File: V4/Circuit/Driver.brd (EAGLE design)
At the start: 58.1 x 81.3 mm, 54 parts, among them IC1 DRV8303DCA

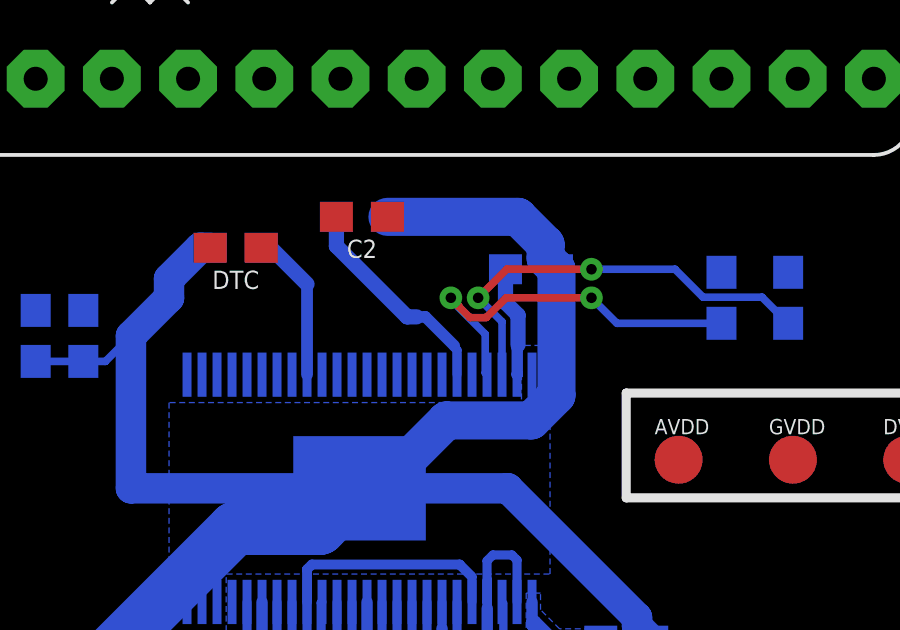
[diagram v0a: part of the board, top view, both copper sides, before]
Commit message: Ready for V4 autoroutering 4
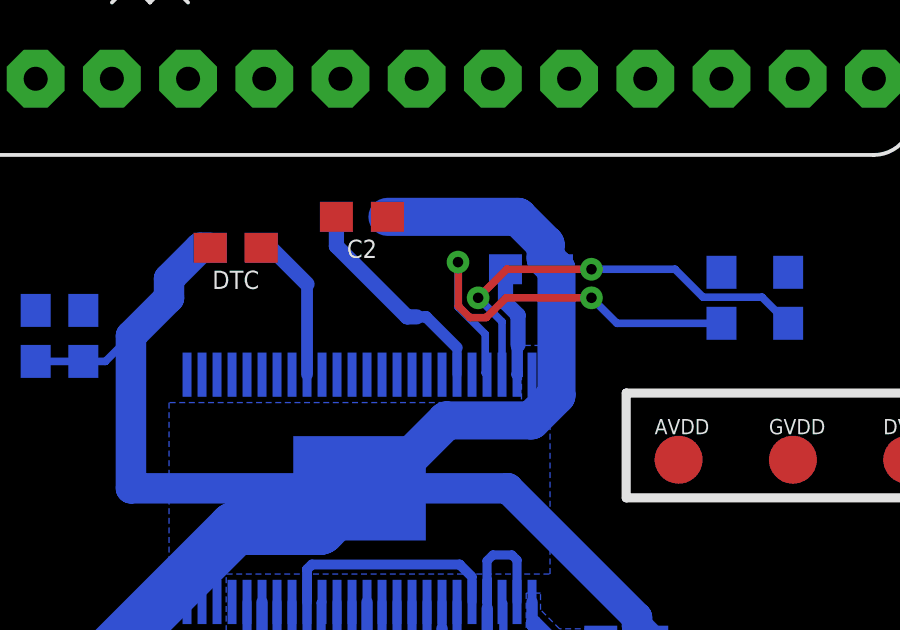
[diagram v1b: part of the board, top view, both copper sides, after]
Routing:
- net SO1B: track 13.0 -> 15.2 mm
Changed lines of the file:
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@@
 <wire x1="34.789375" y1="57.30875" x2="34.789375" y2="56.333125" width="0.508" layer="16"/>
 <wire x1="37.1475" y1="53.975" x2="37.465" y2="53.975" width="0.508" layer="16"/>
-<wire x1="38.694525" y1="52.982025" x2="38.81" y2="52.86655" width="0.3048" layer="16"/>
-<wire x1="38.81" y1="52.86655" x2="38.81" y2="52.048" width="0.3048" layer="16"/>
 <wire x1="34.789375" y1="56.333125" x2="37.1475" y2="53.975" width="0.508" layer="16"/>
-<wire x1="37.465" y1="53.975" x2="37.75543125" y2="53.975" width="0.381" layer="16"/>
-<wire x1="37.75543125" y1="53.975" x2="38.721465625" y2="53.008965625" width="0.381" layer="16"/>
+<wire x1="37.465" y1="53.975" x2="37.7825" y2="53.975" width="0.381" layer="16"/>
+<wire x1="38.81" y1="52.9475" x2="38.81" y2="52.048" width="0.3048" layer="16"/>
+<wire x1="37.7825" y1="53.975" x2="38.81" y2="52.9475" width="0.381" layer="16"/>
 <wire x1="38.81" y1="52.048" x2="53.81625" y2="49.2125" width="0" layer="19" extent="1-16"/>
-<wire x1="38.721465625" y1="53.008965625" x2="38.694525" y2="52.982025" width="0" layer="19" extent="16-16"/>
 </signal>
 <signal name="SO1">
@@
 <contactref element="IC1" pad="21"/>
 <contactref element="R5" pad="2"/>
-<via x="38.60425625" y="54.61" extent="1-16" drill="0.35"/>
-<wire x1="38.60425625" y1="54.5450625" x2="38.60425625" y2="54.61" width="0.254" layer="16"/>
-<wire x1="39.7498" y1="53.39951875" x2="38.60425625" y2="54.5450625" width="0.254" layer="16"/>
+<via x="38.84238125" y="55.800625" extent="1-16" drill="0.35"/>
+<wire x1="38.84238125" y1="54.3069375" x2="38.84238125" y2="55.800625" width="0.254" layer="16"/>
+<wire x1="39.7498" y1="53.39951875" x2="38.84238125" y2="54.3069375" width="0.254" layer="16"/>
 <wire x1="39.81" y1="52.048" x2="39.7498" y2="52.1082" width="0.254" layer="16"/>
 <wire x1="39.7498" y1="52.1082" x2="39.7498" y2="53.39951875" width="0.254" layer="16"/>
@@
 <wire x1="39.24066875" y1="53.9524" x2="38.85545625" y2="54.3376125" width="0.254" layer="1"/>
 <wire x1="43.2906" y1="54.61" x2="40.44304375" y2="54.61" width="0.254" layer="1"/>
-<wire x1="38.85545625" y1="54.3376125" x2="38.85545625" y2="54.3588" width="0.254" layer="1"/>
-<wire x1="38.85545625" y1="54.3588" x2="38.60425625" y2="54.61" width="0.254" layer="1"/>
+<wire x1="38.85545625" y1="54.3376125" x2="38.85545625" y2="55.78755" width="0.254" layer="1"/>
+<wire x1="38.85545625" y1="55.78755" x2="38.84238125" y2="55.800625" width="0.254" layer="1"/>
 <wire x1="40.44304375" y1="54.61" x2="39.78544375" y2="53.9524" width="0.254" layer="1"/>
 </signal>

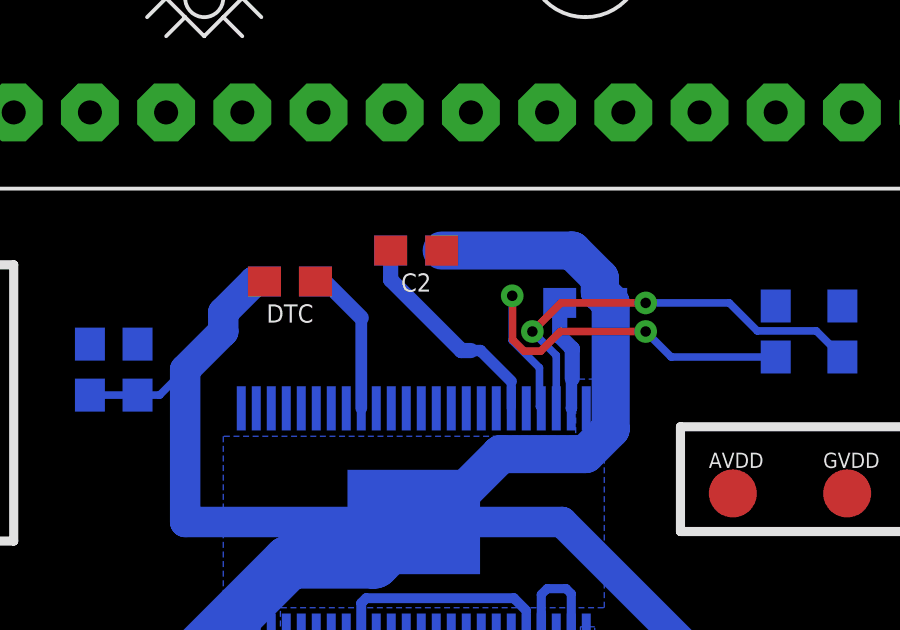
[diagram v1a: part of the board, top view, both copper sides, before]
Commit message: Ready for V4 autoroutering 5
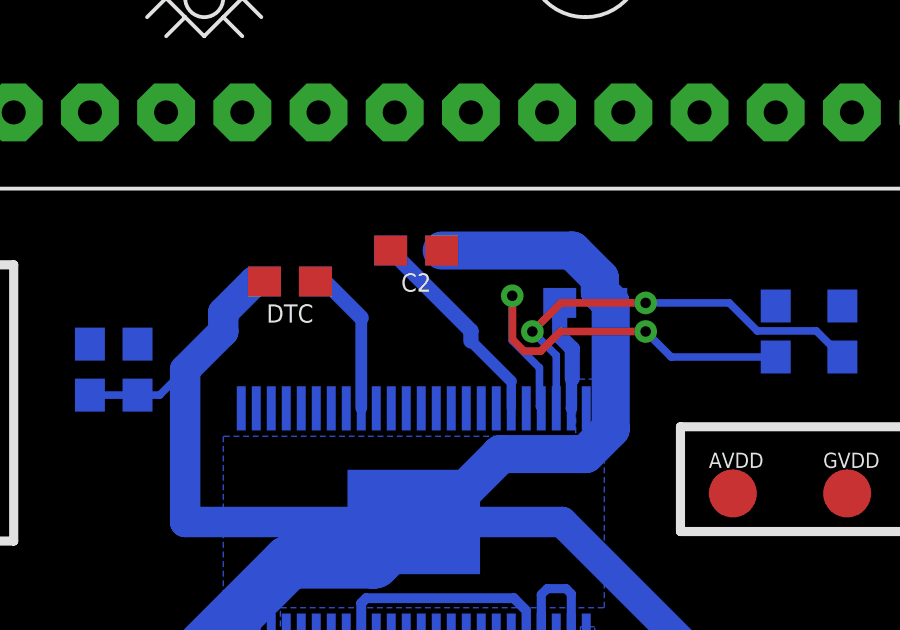
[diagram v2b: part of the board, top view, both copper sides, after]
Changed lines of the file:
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@@
 <wire x1="36.489375" y1="57.30875" x2="40.8423" y2="57.30875" width="1.27" layer="16"/>
 <wire x1="40.8423" y1="57.30875" x2="41.7624" y2="56.38865" width="1.27" layer="16"/>
-<wire x1="42.125" y1="55.5625" x2="50.165" y2="61.9125" width="0" layer="19" extent="16-16"/>
-<wire x1="32.2825" y1="56.276875" x2="30.5825" y2="56.276875" width="0" layer="19" extent="1-16"/>
-<wire x1="3.568" y1="55.245" x2="9.31" y2="39.37" width="0" layer="19" extent="1-1"/>
-<wire x1="4.445" y1="77.1525" x2="3.568" y2="55.245" width="0" layer="19" extent="1-1"/>
-<wire x1="6.985" y1="77.1525" x2="4.445" y2="77.1525" width="0" layer="19" extent="1-1"/>
 </signal>
 <signal name="N$4">
@@
 <contactref element="IC1" pad="45"/>
 <contactref element="IC1" pad="20"/>
-<wire x1="39.31" y1="52.048" x2="52.705" y2="61.9125" width="0" layer="19" extent="16-16"/>
-<wire x1="31.31" y1="44.472" x2="39.31" y2="52.048" width="0" layer="19" extent="16-16"/>
-<wire x1="9.525" y1="77.1525" x2="39.31" y2="52.048" width="0" layer="19" extent="16-16"/>
 </signal>
 <signal name="N$6">
@@
 <wire x1="28.2575" y1="26.035" x2="28.2575" y2="24.9875" width="0.3048" layer="1"/>
 <wire x1="28.2575" y1="24.9875" x2="26.41" y2="23.14" width="0.3048" layer="1"/>
-<wire x1="24.13" y1="2.54" x2="24.13" y2="3.175" width="0" layer="19" extent="1-1"/>
 </signal>
 <signal name="GL_A">
@@
 <contactref element="U$1" pad="P$3"/>
 <contactref element="N_OCTW" pad="TP"/>
-<wire x1="26.3525" y1="54.19" x2="29.81" y2="52.048" width="0" layer="19" extent="16-16"/>
-<wire x1="20.0025" y1="48.815625" x2="26.3525" y2="54.19" width="0" layer="19" extent="1-16"/>
-<wire x1="9.525" y1="61.9125" x2="20.0025" y2="48.815625" width="0" layer="19" extent="1-1"/>
 </signal>
 <signal name="N_FAULT">
@@
 <contactref element="N_FAULT" pad="TP"/>
 <wire x1="7.2" y1="61.9125" x2="6.985" y2="61.9125" width="0.254" layer="16"/>
-<wire x1="24.765" y1="54.19" x2="30.31" y2="52.048" width="0" layer="19" extent="16-16"/>
-<wire x1="9.68375" y1="48.895" x2="24.765" y2="54.19" width="0" layer="19" extent="1-16"/>
-<wire x1="7.2" y1="61.9125" x2="9.68375" y2="48.895" width="0" layer="19" extent="1-16"/>
 </signal>
 <signal name="NSCS">
 <contactref element="IC1" pad="4"/>
 <contactref element="U$1" pad="P$32"/>
-<wire x1="31.31" y1="52.048" x2="32.385" y2="77.1525" width="0" layer="19" extent="16-16"/>
 </signal>
 <signal name="SDI">
 <contactref element="IC1" pad="5"/>
 <contactref element="U$1" pad="P$29"/>
-<wire x1="31.81" y1="52.048" x2="24.765" y2="77.1525" width="0" layer="19" extent="16-16"/>
 </signal>
 <signal name="SDO">
 <contactref element="IC1" pad="6"/>
 <contactref element="U$1" pad="P$30"/>
-<wire x1="32.31" y1="52.048" x2="27.305" y2="77.1525" width="0" layer="19" extent="16-16"/>
 </signal>
 <signal name="SCLK">
 <contactref element="IC1" pad="7"/>
 <contactref element="U$1" pad="P$31"/>
-<wire x1="32.81" y1="52.048" x2="29.845" y2="77.1525" width="0" layer="19" extent="16-16"/>
 </signal>
 <signal name="DC_CAL">
 <contactref element="IC1" pad="8"/>
 <contactref element="U$1" pad="P$12"/>
-<wire x1="33.31" y1="52.048" x2="32.385" y2="61.9125" width="0" layer="19" extent="16-16"/>
 </signal>
 <signal name="GVDD">
@@
 <wire x1="33.81" y1="55.066875" x2="32.6" y2="56.276875" width="0.508" layer="16"/>
 <wire x1="32.2825" y1="56.276875" x2="32.6" y2="56.276875" width="0.508" layer="16"/>
-<wire x1="33.81" y1="52.048" x2="50.00625" y2="49.2125" width="0" layer="19" extent="1-16"/>
 </signal>
 <signal name="N$35">
 <contactref element="IC1" pad="10"/>
 <contactref element="C2" pad="2"/>
-<wire x1="34.31" y1="52.048" x2="34.789375" y2="57.30875" width="0" layer="19" extent="1-16"/>
 </signal>
 <signal name="N$36">
 <contactref element="IC1" pad="11"/>
 <contactref element="C2" pad="1"/>
-<wire x1="34.81" y1="52.048" x2="36.489375" y2="57.30875" width="0" layer="19" extent="1-16"/>
 </signal>
 <signal name="EN_GATE">
@@
 <contactref element="D1" pad="C"/>
 <contactref element="U$1" pad="P$1"/>
-<wire x1="5.322" y1="55.245" x2="35.31" y2="52.048" width="0" layer="19" extent="1-16"/>
-<wire x1="4.445" y1="61.9125" x2="5.322" y2="55.245" width="0" layer="19" extent="1-1"/>
 </signal>
 <signal name="INHA">
@@
 <contactref element="INHA" pad="TP"/>
 <contactref element="U$1" pad="P$5"/>
-<wire x1="14.605" y1="61.9125" x2="35.81" y2="52.048" width="0" layer="19" extent="16-16"/>
-<wire x1="9.525" y1="54.9275" x2="14.605" y2="61.9125" width="0" layer="19" extent="1-1"/>
 </signal>
 <signal name="INLA">
 <contactref element="IC1" pad="14"/>
 <contactref element="U$1" pad="P$14"/>
-<wire x1="36.31" y1="52.048" x2="37.465" y2="61.9125" width="0" layer="19" extent="16-16"/>
 </signal>
 <signal name="INHB">
@@
 <contactref element="INHB" pad="TP"/>
 <contactref element="U$1" pad="P$6"/>
-<wire x1="17.145" y1="61.9125" x2="36.81" y2="52.048" width="0" layer="19" extent="16-16"/>
-<wire x1="14.605" y1="54.9275" x2="17.145" y2="61.9125" width="0" layer="19" extent="1-1"/>
 </signal>
 <signal name="INLB">
 <contactref element="IC1" pad="16"/>
 <contactref element="U$1" pad="P$15"/>
-<wire x1="37.31" y1="52.048" x2="40.005" y2="61.9125" width="0" layer="19" extent="16-16"/>
 </signal>
 <signal name="INHC">
@@
 <contactref element="INHC" pad="TP"/>
 <contactref element="U$1" pad="P$7"/>
-<wire x1="20.0025" y1="54.9275" x2="37.81" y2="52.048" width="0" layer="19" extent="1-16"/>
-<wire x1="19.685" y1="61.9125" x2="20.0025" y2="54.9275" width="0" layer="19" extent="1-1"/>
 </signal>
 <signal name="INLC">
 <contactref element="IC1" pad="18"/>
 <contactref element="U$1" pad="P$16"/>
-<wire x1="38.31" y1="52.048" x2="42.545" y2="61.9125" width="0" layer="19" extent="16-16"/>
 </signal>
 <signal name="DVDD">
@@
 <contactref element="DVDD_CAP" pad="1"/>
 <contactref element="DVDD" pad="TP"/>
-<wire x1="34.789375" y1="57.30875" x2="34.789375" y2="56.333125" width="0.508" layer="16"/>
-<wire x1="37.1475" y1="53.975" x2="37.465" y2="53.975" width="0.508" layer="16"/>
-<wire x1="34.789375" y1="56.333125" x2="37.1475" y2="53.975" width="0.508" layer="16"/>
-<wire x1="37.465" y1="53.975" x2="37.7825" y2="53.975" width="0.381" layer="16"/>
 <wire x1="38.81" y1="52.9475" x2="38.81" y2="52.048" width="0.3048" layer="16"/>
-<wire x1="37.7825" y1="53.975" x2="38.81" y2="52.9475" width="0.381" layer="16"/>
+<wire x1="37.465" y1="54.2925" x2="38.81" y2="52.9475" width="0.381" layer="16"/>
+<wire x1="34.789375" y1="57.30875" x2="37.465" y2="54.633125" width="0.508" layer="16"/>
+<wire x1="37.465" y1="54.633125" x2="37.465" y2="54.2925" width="0.508" layer="16"/>
 <wire x1="38.81" y1="52.048" x2="53.81625" y2="49.2125" width="0" layer="19" extent="1-16"/>
 </signal>
@@
 <contactref element="U$1" pad="P$8"/>
 <contactref element="R5" pad="1"/>
-<wire x1="22.225" y1="61.9125" x2="47.625" y2="55.46" width="0" layer="19" extent="16-16"/>
 </signal>
 <signal name="SO2">
@@
 <contactref element="R6" pad="1"/>
 <wire x1="24.765" y1="61.9125" x2="25.0825" y2="61.9125" width="0.254" layer="16"/>
-<wire x1="25.0825" y1="61.9125" x2="49.8475" y2="55.46" width="0" layer="19" extent="16-16"/>
 </signal>
 <signal name="GH_B">
@@
 <contactref element="DTC" pad="2"/>
 <contactref element="IC1" pad="3"/>
-<wire x1="30.81" y1="52.048" x2="30.5825" y2="56.276875" width="0" layer="19" extent="1-16"/>
 </signal>
 <signal name="AVDD">
@@
 <wire x1="40.8171" y1="52.92753125" x2="40.8171" y2="52.0551" width="0.381" layer="16"/>
 <wire x1="40.8171" y1="52.0551" x2="40.81" y2="52.048" width="0.381" layer="16"/>
-<wire x1="40.81" y1="52.048" x2="46.19625" y2="49.2125" width="0" layer="19" extent="1-16"/>
 </signal>
 <signal name="N$3">
